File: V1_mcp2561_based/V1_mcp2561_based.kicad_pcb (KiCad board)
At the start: 2 copper layers, 12 parts, among them J1 Screw_Terminal_01x03, U1 RP2040, U2 MCP2561-E-P, U3 ESP32-S3-DevKitC

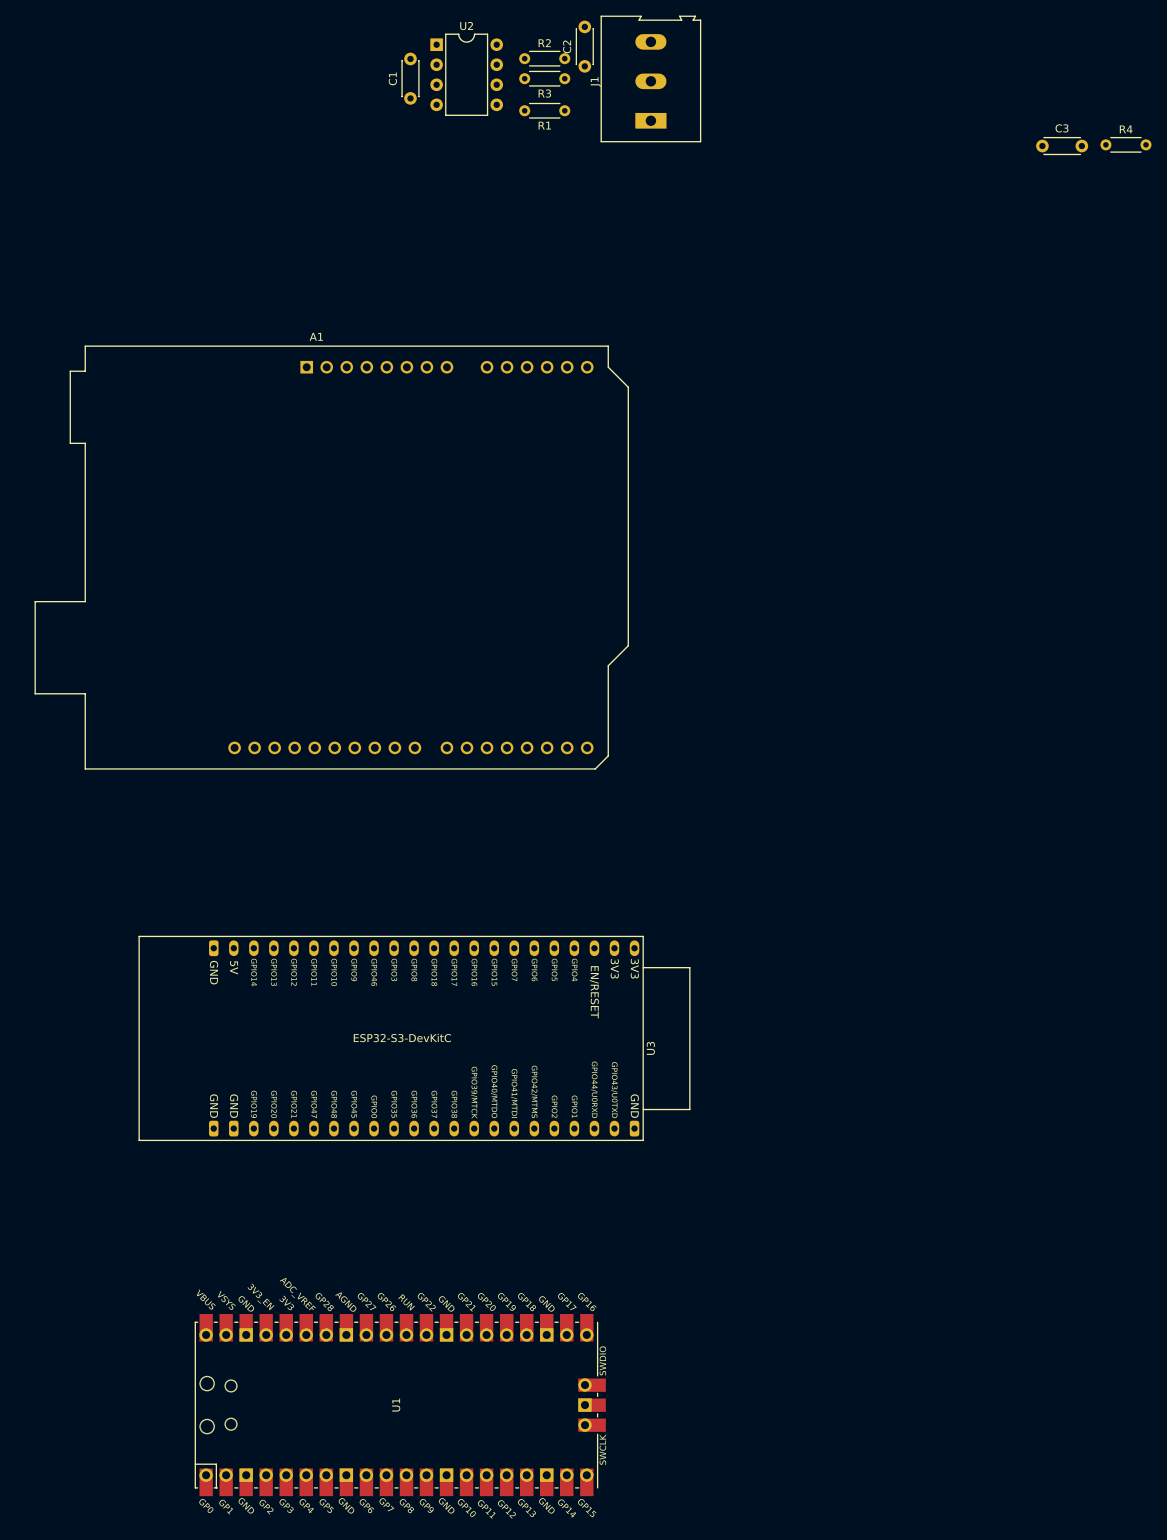
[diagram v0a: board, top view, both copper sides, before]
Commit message: e
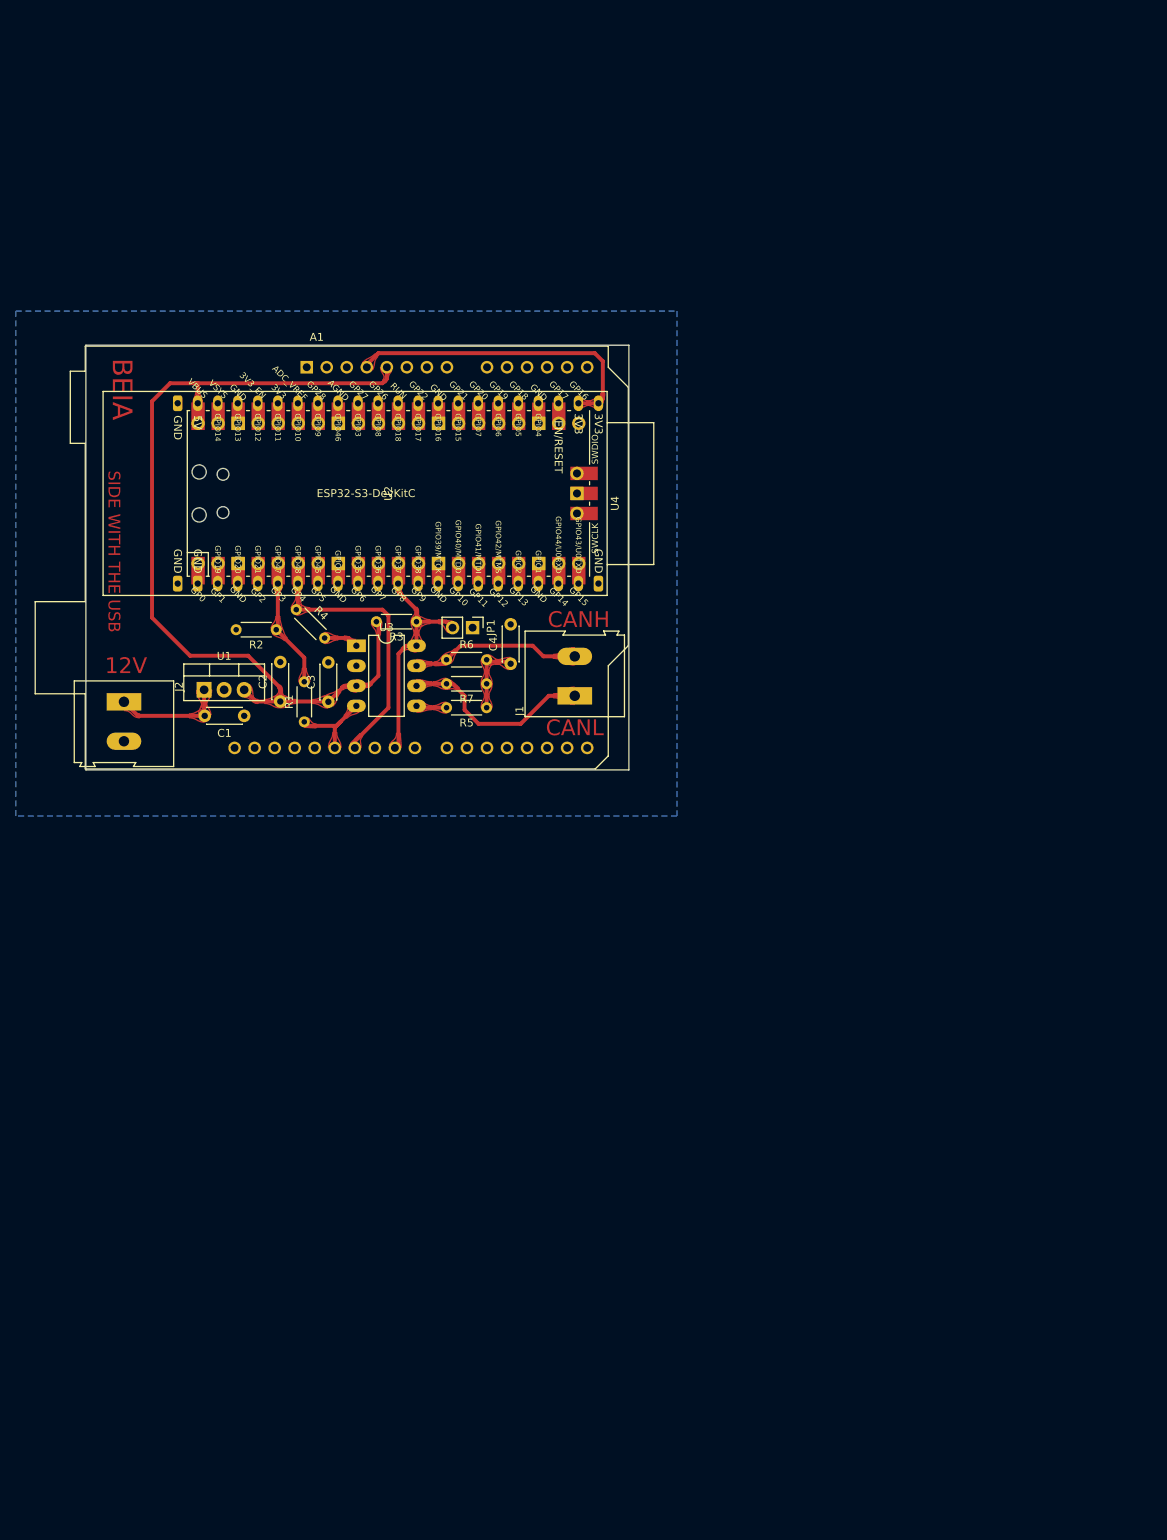
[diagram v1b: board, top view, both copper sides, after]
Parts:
- removed the C3 at (188.1, 50.7)
- added C1: C_Small, Capacitor_THT:C_Disc_D4.3mm_W1.9mm_P5.00mm, F.Cu at (86.9, 122.9)
- added C2: C_Small, Capacitor_THT:C_Disc_D4.3mm_W1.9mm_P5.00mm, F.Cu at (91.4, 121.1)
- added J2: Screw_Terminal_01x02, TerminalBlock:TerminalBlock_Altech_AK300-2_P5.00mm, F.Cu at (71.6, 121.2)
- added JP1: Jumper_2_Bridged, Connector_PinHeader_2.54mm:PinHeader_1x02_P2.54mm_Vertical, F.Cu at (115.8, 111.8)
- added R1: R_Small, Resistor_THT:R_Axial_DIN0204_L3.6mm_D1.6mm_P5.08mm_Horizontal, F.Cu at (94.5, 123.7)
- added R2: R_Small, Resistor_THT:R_Axial_DIN0204_L3.6mm_D1.6mm_P5.08mm_Horizontal, F.Cu at (90.9, 112.0)
- added R3: 10k, Resistor_THT:R_Axial_DIN0204_L3.6mm_D1.6mm_P5.08mm_Horizontal, F.Cu at (108.7, 111.0)
- added U2: RP2040, MCU_RaspberryPi_and_Boards:RPi_Pico_SMD_TH, F.Cu at (105.2, 94.7)
- J1: value Screw_Terminal_01x03 -> Screw_Terminal_01x02; footprint TerminalBlock:TerminalBlock_Altech_AK300-3_P5.00mm -> TerminalBlock:TerminalBlock_Altech_AK300-2_P5.00mm
- U1: value RP2040 -> LF50_TO220; footprint MCU_RaspberryPi_and_Boards:RPi_Pico_SMD_TH -> Package_TO_SOT_THT:TO-220-3_Vertical
- U3: renamed from U2; footprint Package_DIP:DIP-8_W7.62mm -> Package_DIP:DIP-8_W7.62mm_LongPads
- moved R4 118.3 mm to (93.5, 109.5), turned to -45 degrees
- moved U1 93.9 mm to (81.8, 119.6), turned to 0 degrees
- moved R7 77.3 mm to (117.6, 118.9)
- moved C3 77.2 mm to (97.5, 121.2)
- moved U3 76.9 mm to (101.1, 114.1)
- moved R6 76.8 mm to (112.5, 115.8)
- moved R5 76.3 mm to (117.6, 121.9)
- moved C4 76.3 mm to (120.7, 116.3)
- moved J1 73.5 mm to (128.8, 120.4)
- moved U4 69.2 mm to (131.8, 83.3)
- renumbered C1 to C3, C2 to C4, R1 to R5, R2 to R6, R3 to R7, U3 to U4
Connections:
- A1 pad 24: unconnected-(A1-Pad24) -> /STBY
- A1 pad 26: unconnected-(A1-Pad26) -> /TX-pin
- A1 pad 27: unconnected-(A1-Pad27) -> /RXD
- A1 pad 4: unconnected-(A1-Pad4) -> +3V3
- J1 pad 2: GND -> /CANH
- R4 pad 1: unconnected-(R4-Pad1) -> /TX-pin
- R4 pad 2: unconnected-(R4-Pad2) -> /TXD
- U1 pad 1: unconnected-(U1-Pad1) -> +12V
- U1 pad 2: unconnected-(U1-Pad2) -> GND
- U1 pad 3: unconnected-(U1-Pad3) -> +5V
- U3 pad 1: unconnected-(U2-Pad1) -> /TXD
- U3 pad 4: unconnected-(U2-Pad4) -> /RXD
- U3 pad 8: unconnected-(U2-Pad8) -> /STBY
- U4 pad 28: unconnected-(U3-Pad28) -> /RX-pin
- U4 pad 29: unconnected-(U3-Pad29) -> /TX-pin
- U4 pad 34: unconnected-(U3-Pad34) -> /STBY
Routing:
- net +5V: track 0.00 -> 110.0 mm
- net +3V3: track 0.00 -> 39.4 mm
- net /TX-pin: track 0.00 -> 33.9 mm
- net /STBY: track 0.00 -> 28.6 mm
- net /CANL: track 0.00 -> 24.8 mm
- net /CANH: track 0.00 -> 21.7 mm
- net +12V: track 0.00 -> 14.3 mm
- net /RX-pin: track 0.00 -> 14.0 mm
- net /RXD: track 0.00 -> 11.5 mm
- net Net-(C4-Pad1): track 0.00 -> 9.34 mm
- net /TXD: track 0.00 -> 4.44 mm
- net /SPL: track 0.00 -> 3.90 mm
- added copper zone on B.Cu, net GND
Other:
- board outline added: 68.8 x 53.8 mm
- board text added: "12V"
- board text added: "BEIA"
- board text added: "CANH"
- board text added: "CANL"
- board text added: "SIDE WITH THE USB"

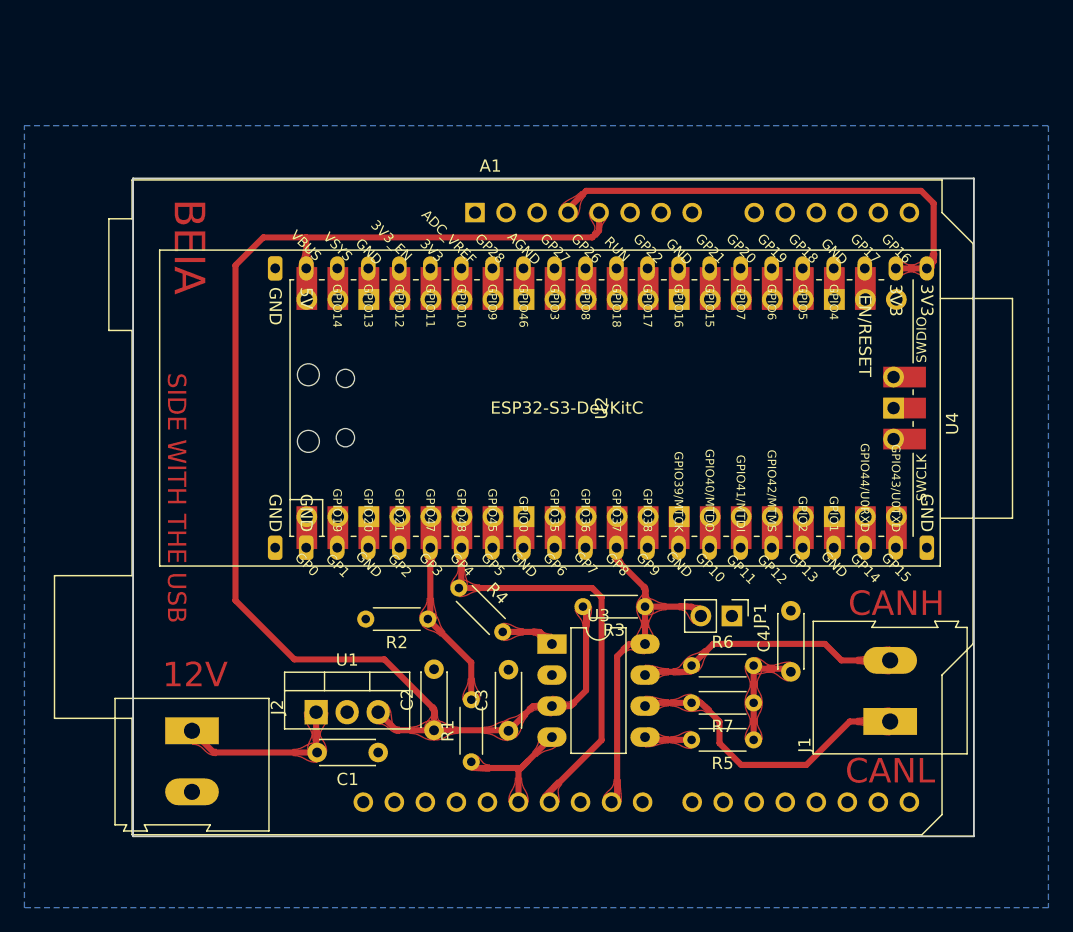
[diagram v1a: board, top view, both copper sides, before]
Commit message: h
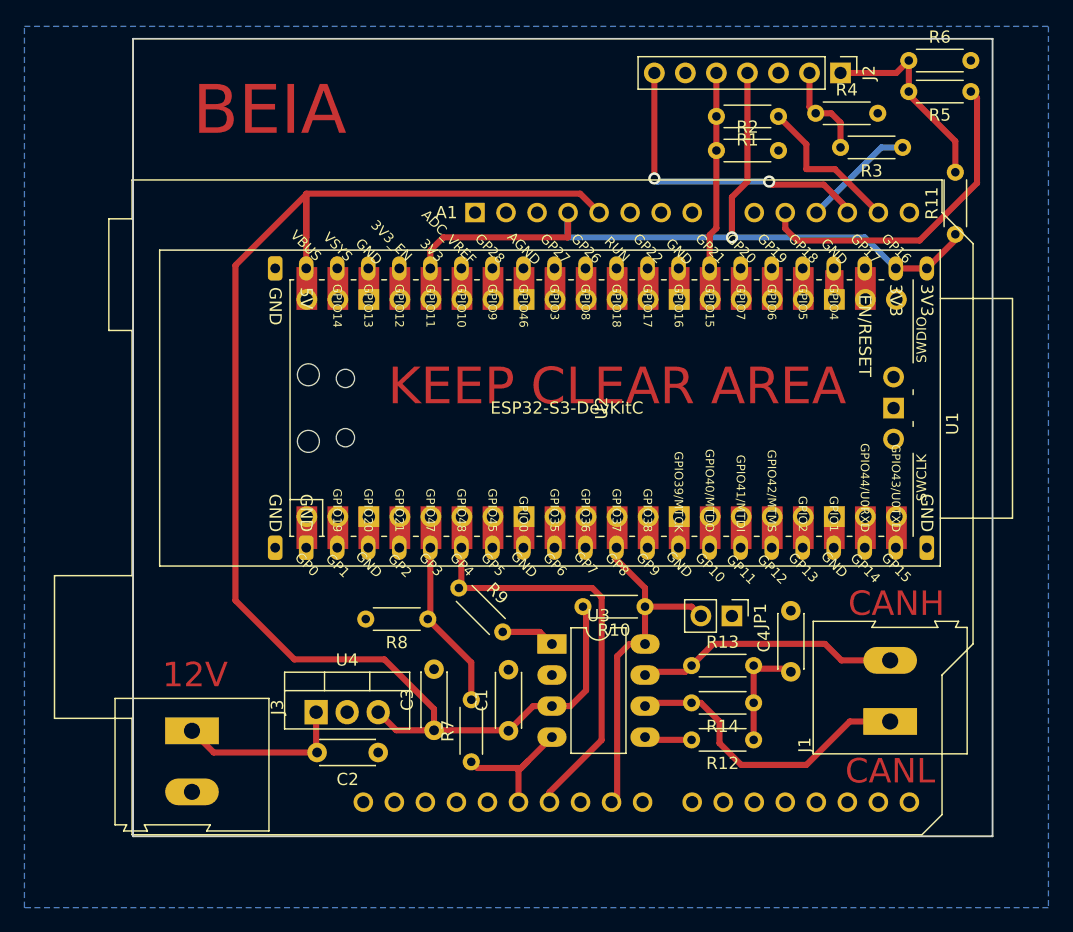
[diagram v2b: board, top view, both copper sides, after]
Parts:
- added J2: Conn_01x07, Connector_PinHeader_2.54mm:PinHeader_1x07_P2.54mm_Vertical, F.Cu at (124.7, 67.3)
- added R1: R_Small, Resistor_THT:R_Axial_DIN0204_L3.6mm_D1.6mm_P5.08mm_Horizontal, F.Cu at (119.6, 70.9)
- added R11: R_Small, Resistor_THT:R_Axial_DIN0204_L3.6mm_D1.6mm_P5.08mm_Horizontal, F.Cu at (134.1, 80.5)
- added R2: R_Small, Resistor_THT:R_Axial_DIN0204_L3.6mm_D1.6mm_P5.08mm_Horizontal, F.Cu at (114.6, 73.7)
- added R3: R_Small, Resistor_THT:R_Axial_DIN0204_L3.6mm_D1.6mm_P5.08mm_Horizontal, F.Cu at (129.8, 73.4)
- added R4: R_Small, Resistor_THT:R_Axial_DIN0204_L3.6mm_D1.6mm_P5.08mm_Horizontal, F.Cu at (122.7, 70.6)
- added R5: R_Small, Resistor_THT:R_Axial_DIN0204_L3.6mm_D1.6mm_P5.08mm_Horizontal, F.Cu at (135.4, 68.8)
- added R6: R_Small, Resistor_THT:R_Axial_DIN0204_L3.6mm_D1.6mm_P5.08mm_Horizontal, F.Cu at (130.3, 66.3)
- renumbered C3 to C1, C1 to C2, C2 to C3, J2 to J3, R3 to R10, R5 to R12, R6 to R13, R7 to R14, R1 to R7, R2 to R8, R4 to R9, U4 to U1, U1 to U4
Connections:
- A1 pad 10: unconnected-(A1-Pad10) -> Net-(A1-Pad10)
- A1 pad 11: unconnected-(A1-Pad11) -> Net-(A1-Pad11)
- A1 pad 12: unconnected-(A1-Pad12) -> /MISO
- A1 pad 13: unconnected-(A1-Pad13) -> Net-(A1-Pad13)
- U1 pad 17: unconnected-(U4-Pad17) -> +3V3
- U1 pad 4: unconnected-(U4-Pad4) -> /MISO
- U1 pad 5: unconnected-(U4-Pad5) -> /SS
- U1 pad 6: unconnected-(U4-Pad6) -> /MOSI
- U1 pad 8: unconnected-(U4-Pad8) -> /CLK
- U2 pad 36: unconnected-(U2-Pad36) -> +3V3
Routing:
- net +3V3: track 39.4 -> 68.0 mm, vias 0 -> 1
- net Net-(A1-Pad10): track 0.00 -> 27.1 mm
- net /MISO: track 0.00 -> 25.8 mm, vias 0 -> 2
- net /SS: track 0.00 -> 16.7 mm
- net /CLK: track 0.00 -> 15.4 mm
- net Net-(A1-Pad13): track 0.00 -> 12.6 mm
- net Net-(A1-Pad11): track 0.00 -> 9.27 mm
- net /MOSI: track 0.00 -> 7.89 mm
- net +5V: track 110.0 -> 117.5 mm
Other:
- board size 68.8 x 53.8 mm -> 70.4 x 65.3 mm
- board text added: "KEEP CLEAR AREA"
- board text removed: "SIDE WITH THE USB"
